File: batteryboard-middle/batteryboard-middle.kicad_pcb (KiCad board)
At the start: 2 copper layers, 46.8 x 46.8 mm, 9 parts, among them J1 FLE-107-01-G-DV-A, J2 Conn_01x02, J3 Conn_01x02, J4 FTS-107-01-L-DV-A

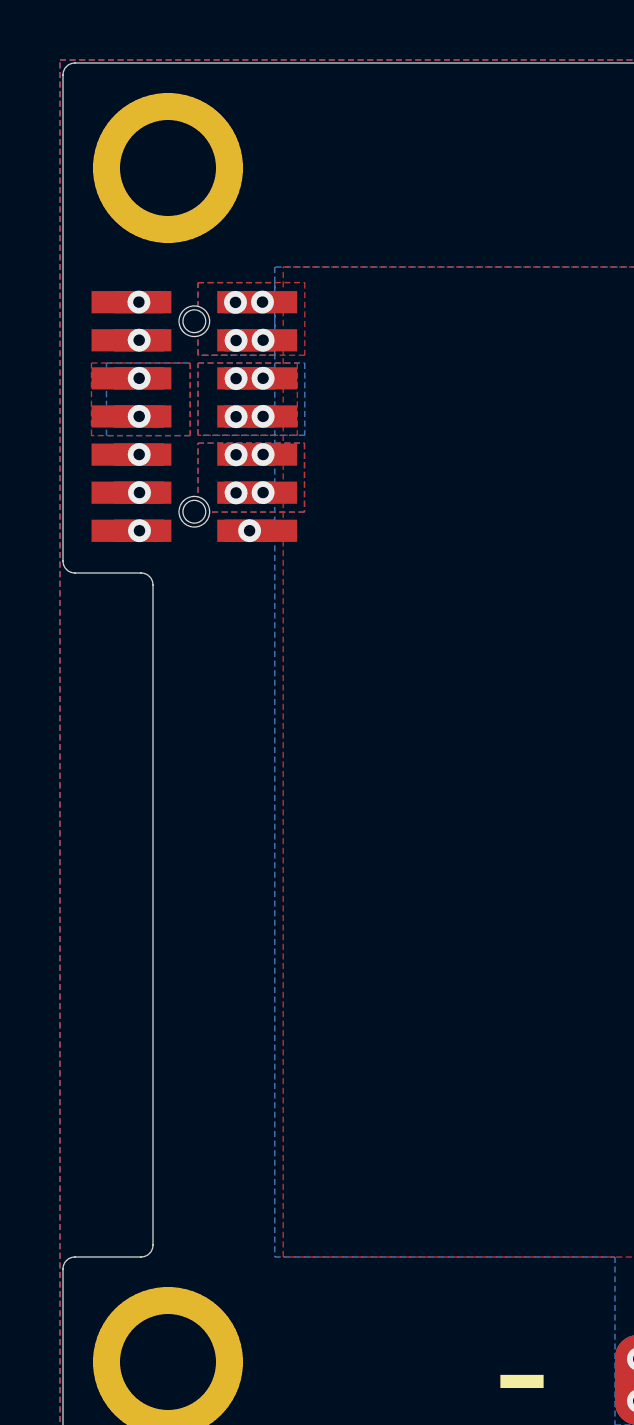
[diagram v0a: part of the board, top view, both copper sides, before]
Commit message: Minor updates and exported STEP / BOM
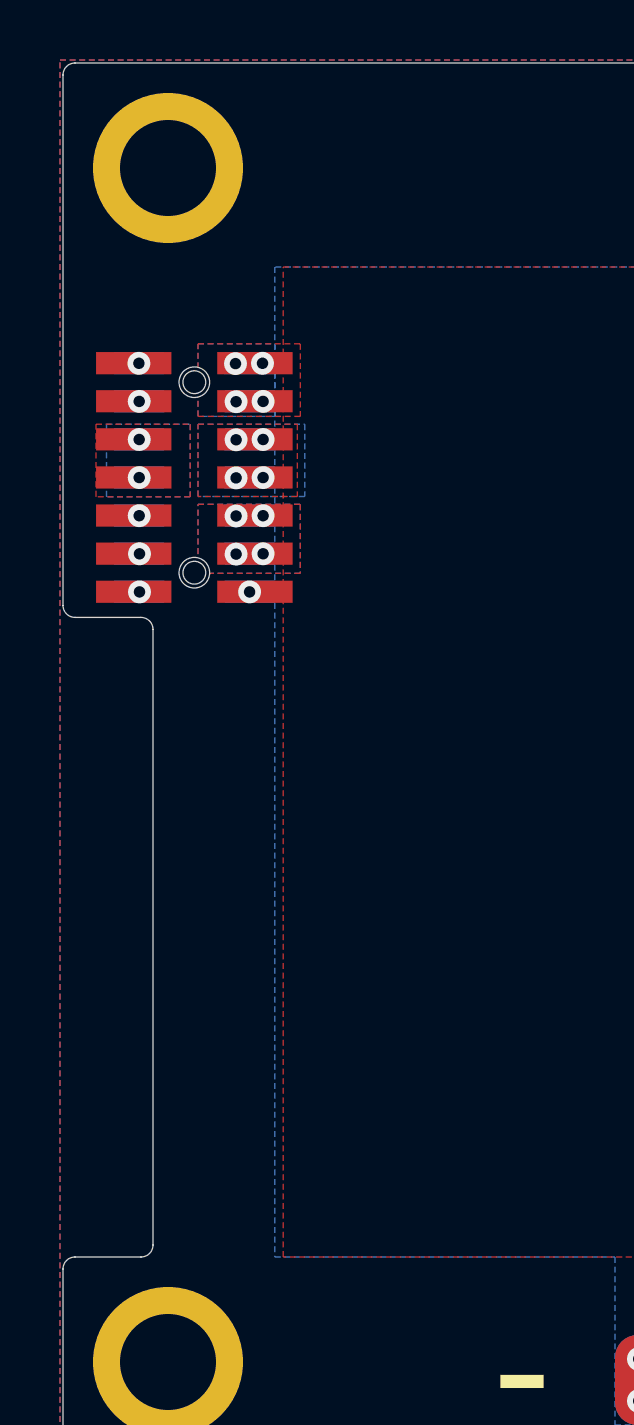
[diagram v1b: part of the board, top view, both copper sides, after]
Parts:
- moved J1 2.03 mm to (127.8, 91.0)
- moved J4 2.03 mm to (127.8, 91.0)
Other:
- outline, holes or cut-outs redrawn
- board text added: "06-NOV-22"
- board text removed: "09-OCT-22"
